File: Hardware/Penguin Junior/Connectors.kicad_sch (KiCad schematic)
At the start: 28 parts, among them J1 USB_B_Micro, J10 Conn_01x06_UART, J10 Conn_01x06_servo, J10 Conn_01x06_servo_5V, J10 Conn_01x06_servo_GND, J11 Conn_01x06_UART, J14 Conn_01x04_UART, J16 Conn_02x05_SWD, J2 Conn_01x03_Video, J2 Micro_SD_Card_Det1, J5 Conn_01x03_Video, J9 Conn_01x04_I2C, U2 USBLC6-2SC6

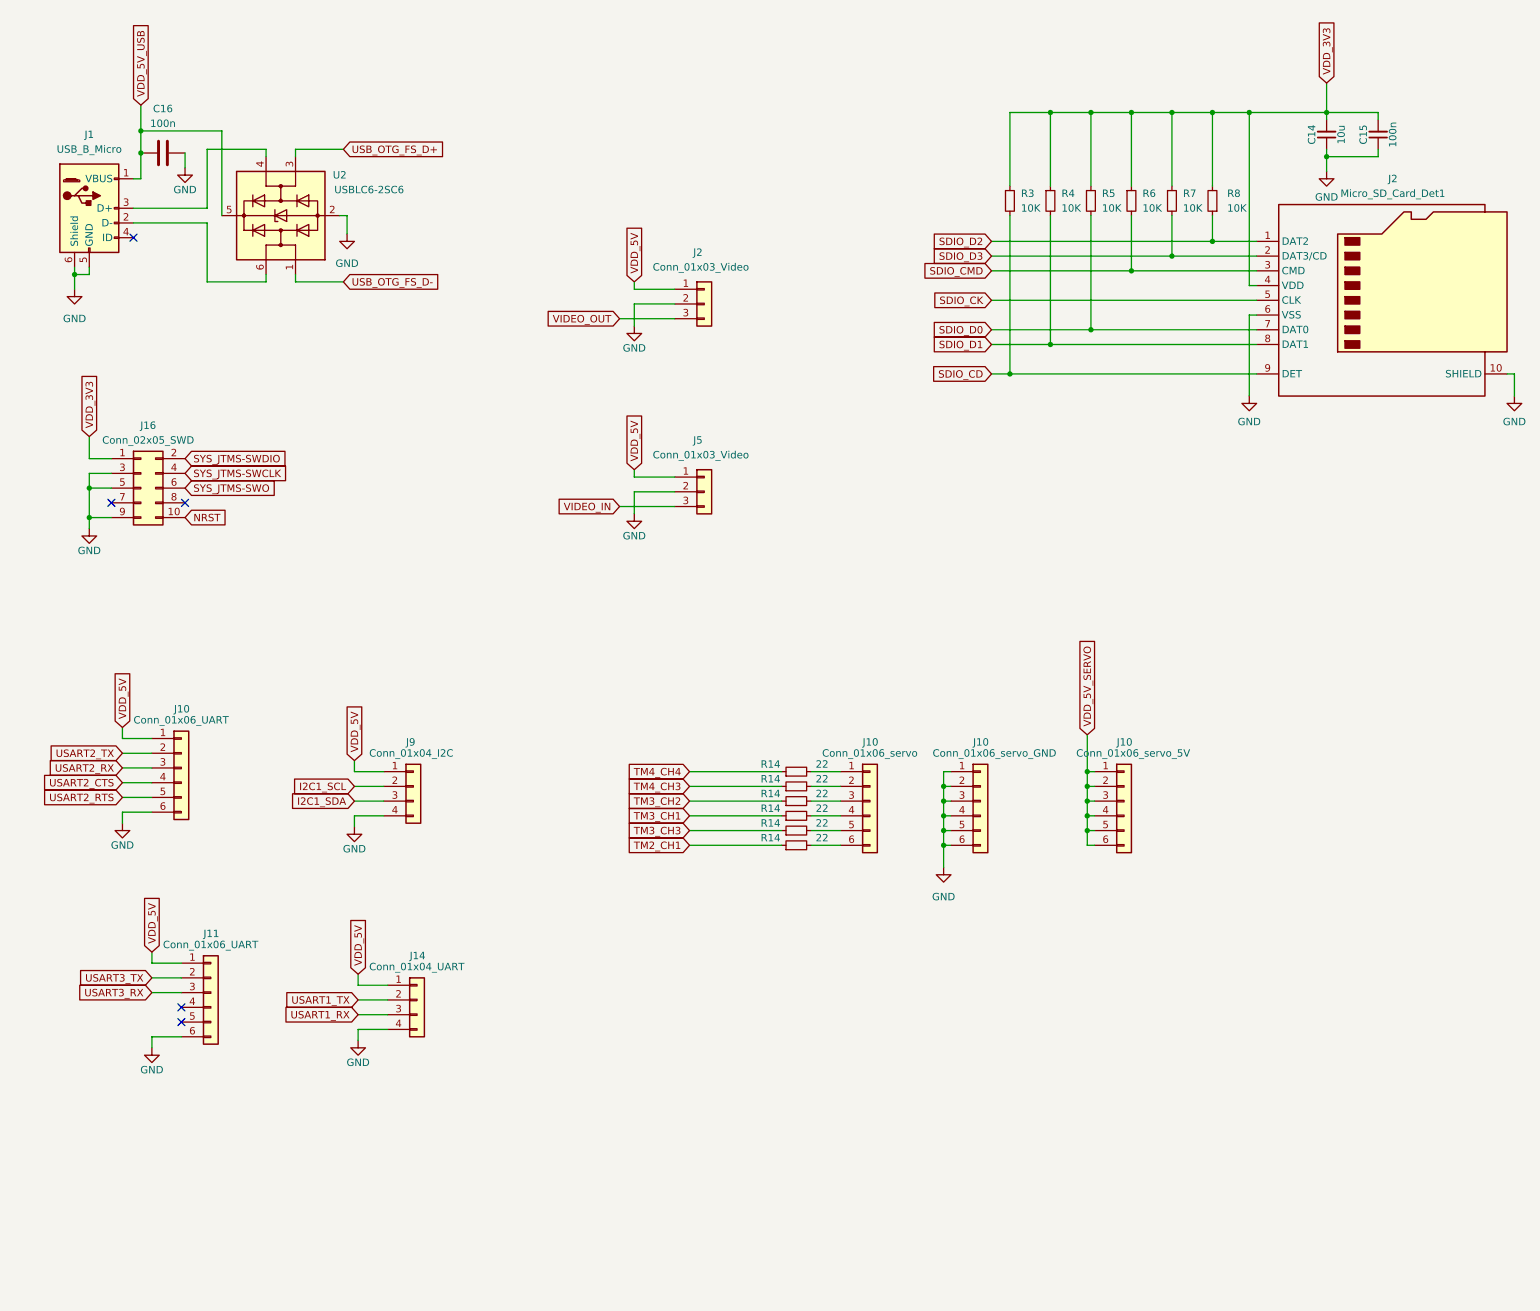
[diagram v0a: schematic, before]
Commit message: Updated project
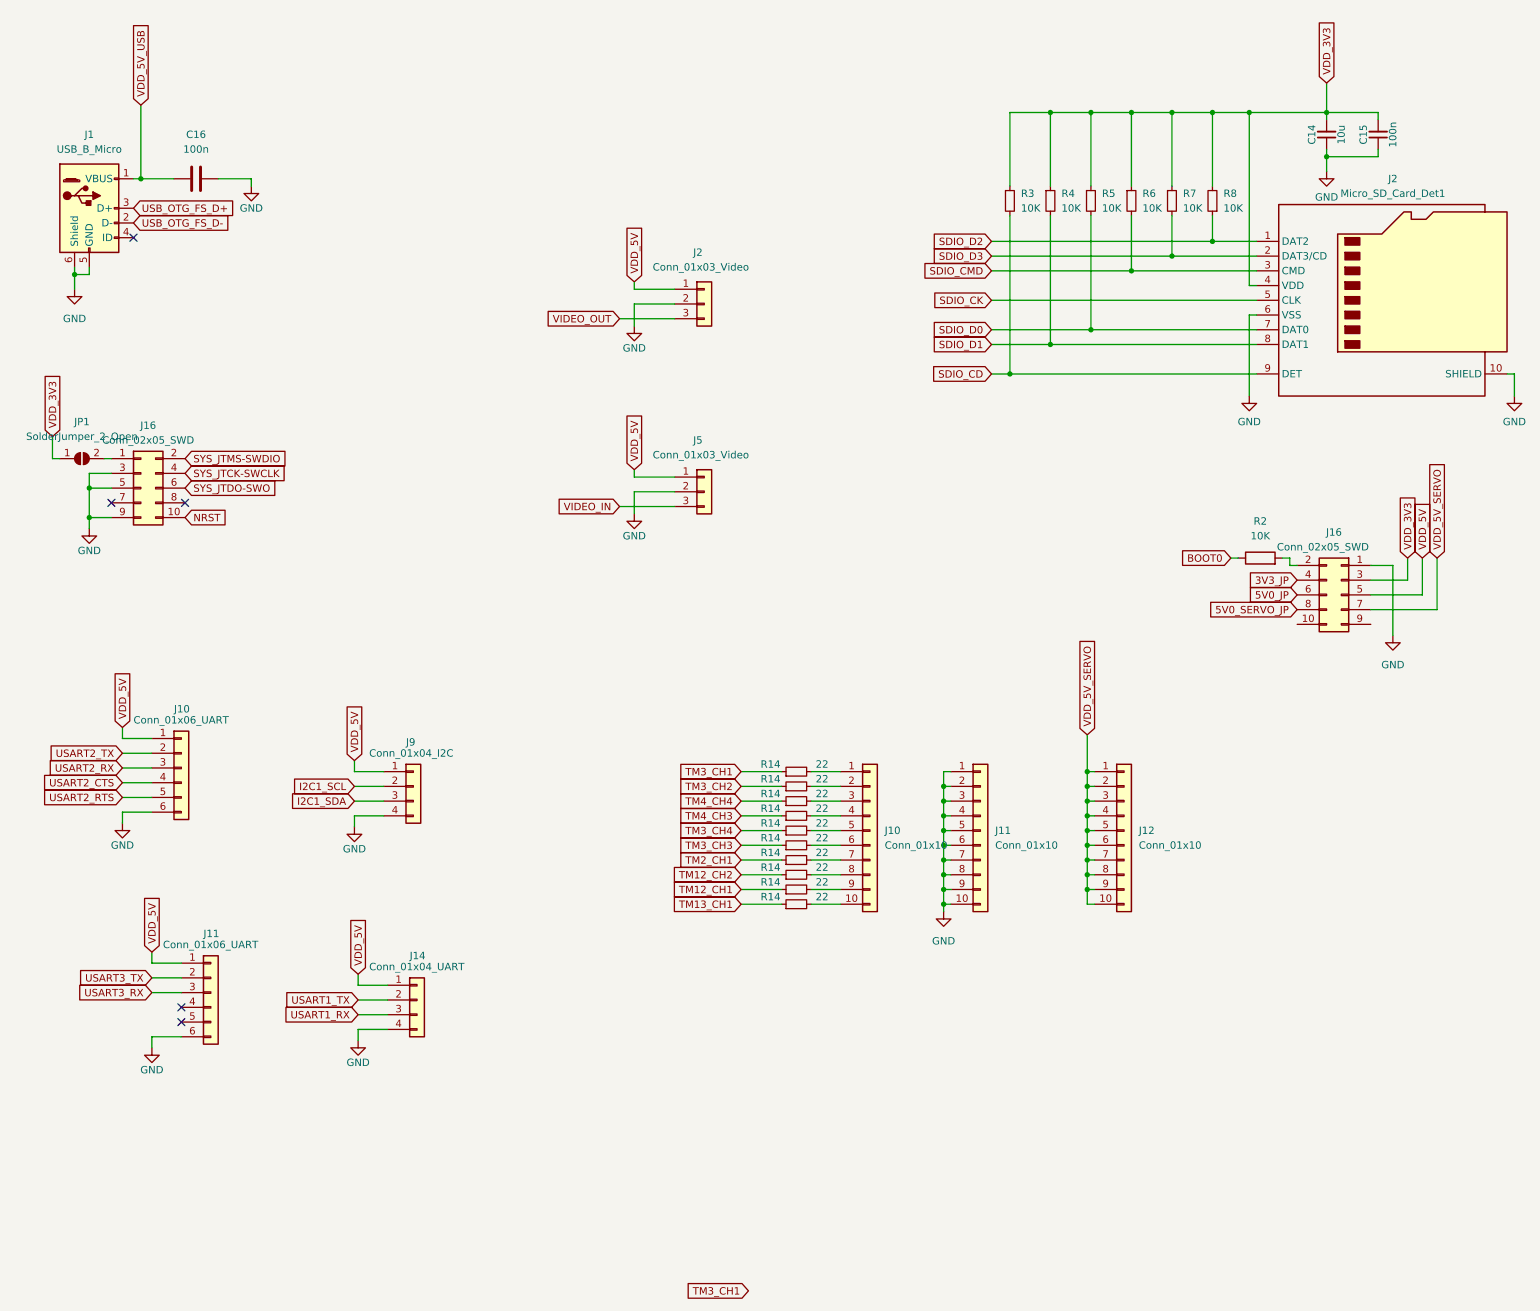
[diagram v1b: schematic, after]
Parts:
- removed J10: Conn_01x06_servo_GND, Connector_PinHeader_2.54mm:PinHeader_1x06_P2.54mm_Vertical, symbol Connector_Generic:Conn_01x06
- removed J10: Conn_01x06_servo, Connector_PinHeader_2.54mm:PinHeader_1x06_P2.54mm_Vertical, symbol Connector_Generic:Conn_01x06
- removed J10: Conn_01x06_servo_5V, Connector_PinHeader_2.54mm:PinHeader_1x06_P2.54mm_Vertical, symbol Connector_Generic:Conn_01x06
- removed U2: USBLC6-2SC6, Package_TO_SOT_SMD:SOT-23-6, symbol Power_Protection:USBLC6-2SC6
- added J10, J11, J12: Conn_01x10, Connector_PinHeader_2.54mm:PinHeader_1x10_P2.54mm_Vertical, symbol Connector_Generic:Conn_01x10
- added J16: Conn_02x05_SWD, Connector_PinHeader_1.27mm:PinHeader_2x05_P1.27mm_Vertical, symbol Connector_Generic:Conn_02x05_Odd_Even
- added JP1: SolderJumper_2_Open, Jumper:SolderJumper-2_P1.3mm_Open_Pad1.0x1.5mm, symbol Jumper:SolderJumper_2_Open
- added R14 (x4): 22, Resistor_SMD:R_0402_1005Metric, symbol Device:R_Small
- added R2: 10K, Resistor_SMD:R_0402_1005Metric, symbol Device:R
- C15, C16: footprint Capacitor_SMD:C_0603_1608Metric -> Capacitor_SMD:C_0402_1005Metric
- R14, R3, R4, R5, R6, R7, R8: footprint Resistor_SMD:R_0603_1608Metric -> Resistor_SMD:R_0402_1005Metric
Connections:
- net GND: now also J11.1 (Pin_1), J11.10 (Pin_10), J11.2 (Pin_2), J11.3 (Pin_3), J11.4 (Pin_4), J11.5 (Pin_5), J11.6 (Pin_6), J11.7 (Pin_7), J11.8 (Pin_8), J11.9 (Pin_9), J16.1 (Pin_1)
- net TM2_CH1: now also R14.1; no longer R14.1
- net TM3_CH1: now also R14.1; no longer R14.1
- net TM3_CH2: now also R14.1; no longer R14.1
- net TM3_CH3: now also R14.1; no longer R14.1
- net TM4_CH3: now also R14.1; no longer R14.1
- net TM4_CH4: now also R14.1; no longer R14.1
- net USB_OTG_FS_D+: now also J1.3 (D+)
- net USB_OTG_FS_D-: now also J1.2 (D-)
- net VDD_3V3: now also J16.3 (Pin_3), JP1.1 (A); no longer J16.1 (Pin_1)
- net VDD_5V: now also J16.5 (Pin_5)
- net VDD_5V_SERVO: now also J12.1 (Pin_1), J12.10 (Pin_10), J12.2 (Pin_2), J12.3 (Pin_3), J12.4 (Pin_4), J12.5 (Pin_5), J12.6 (Pin_6), J12.7 (Pin_7), J12.8 (Pin_8), J12.9 (Pin_9), J16.7 (Pin_7)
- net at R14.2: now also J10.6 (Pin_6)
- net at R14.2: now also J10.3 (Pin_3)
- net at R14.2: now also J10.2 (Pin_2)
- net at R14.2: now also J10.4 (Pin_4)
- net at R14.2: now also J10.1 (Pin_1)
- net at R14.2: now also J10.5 (Pin_5)
- net SYS_JTMS-SWCLK renamed SYS_JTCK-SWCLK
- net SYS_JTMS-SWO renamed SYS_JTDO-SWO
- new net: J10.9 (Pin_9), R14.2
- new net: J16.2 (Pin_2), R2.2
- new net: J10.8 (Pin_8), R14.2
- new net: J16.1 (Pin_1), JP1.2 (B)
- new net: J10.10 (Pin_10), R14.2
- new net: J10.7 (Pin_7), R14.2
- new net 3V3_JP: J16.4 (Pin_4)
- new net 5V0_JP: J16.6 (Pin_6)
- new net 5V0_SERVO_JP: J16.8 (Pin_8)
- new net BOOT0: R2.1
- new net TM12_CH1: R14.1
- new net TM12_CH2: R14.1
- new net TM13_CH1: R14.1
- new net TM3_CH4: R14.1
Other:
- moved on the sheet: C16
